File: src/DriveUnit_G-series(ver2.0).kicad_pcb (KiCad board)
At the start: 2 copper layers, 65.7 x 21.5 mm, 1 part

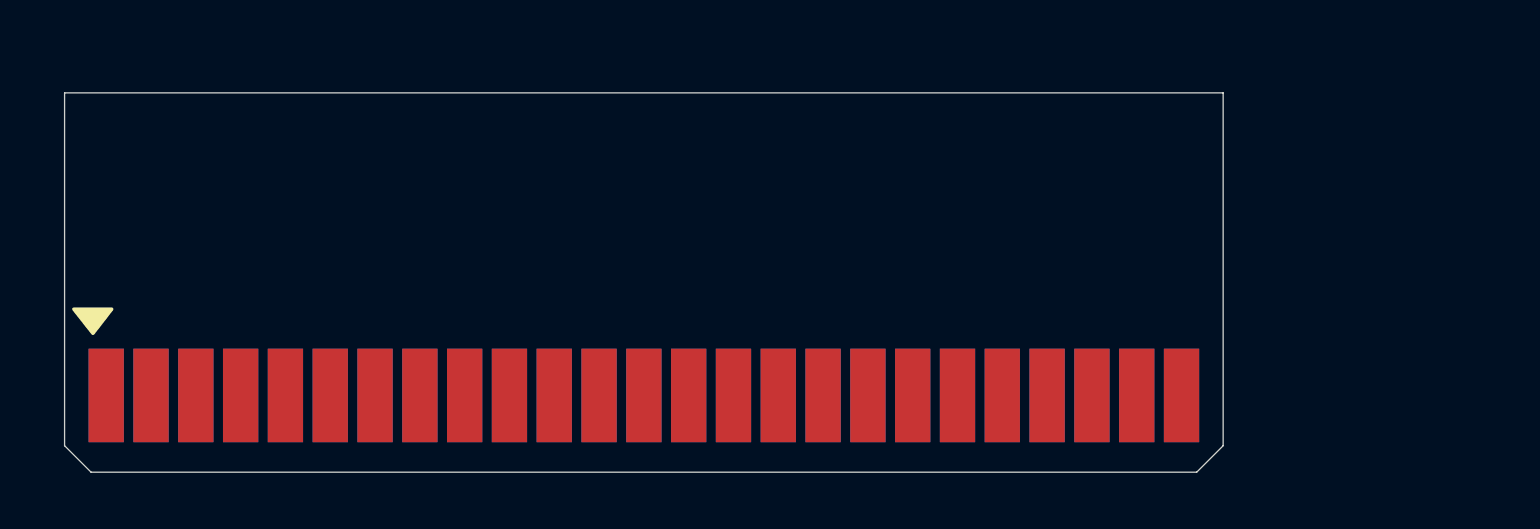
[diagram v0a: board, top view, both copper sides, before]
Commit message: [add]配線途中まで
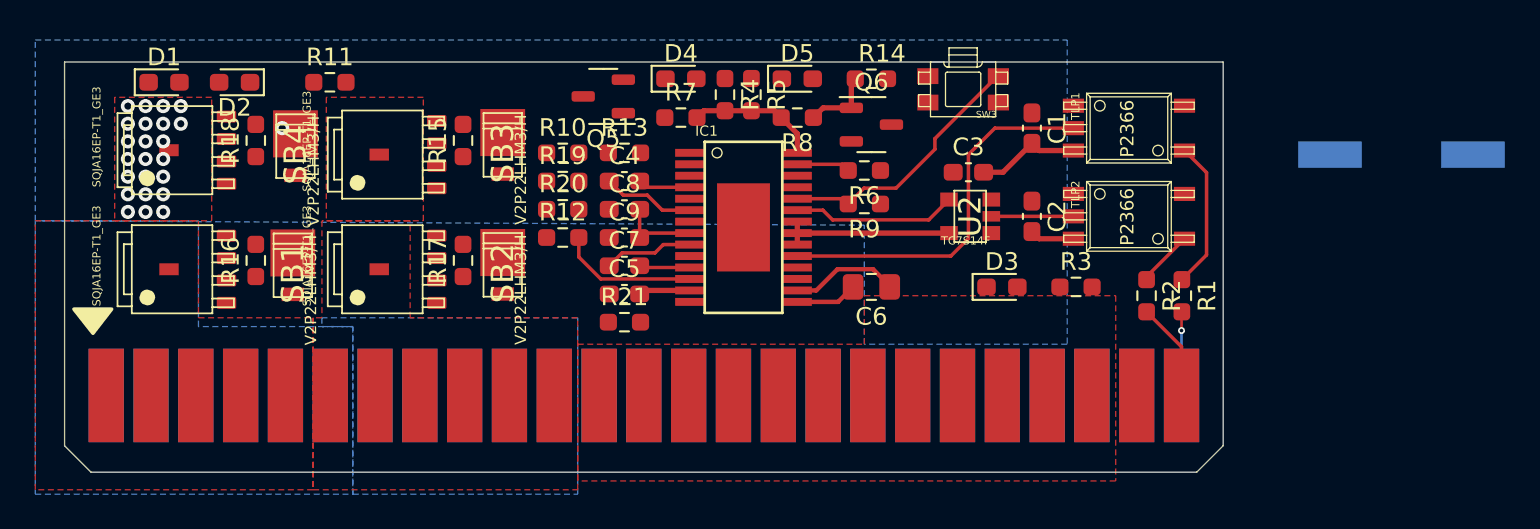
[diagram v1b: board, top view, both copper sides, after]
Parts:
- added C1: 100n, Capacitor_SMD:C_0603_1608Metric_Pad1.08x0.95mm_HandSolder, F.Cu at (170.5, 111.0)
- added C10: 220u, Symbol:U2-R_NCH, B.Cu at (191.4, 112.5)
- added C2: 100n, Capacitor_SMD:C_0603_1608Metric_Pad1.08x0.95mm_HandSolder, F.Cu at (170.5, 116.0)
- added C3: 100n, Capacitor_SMD:C_0603_1608Metric_Pad1.08x0.95mm_HandSolder, F.Cu at (166.9, 113.5)
- added C4: 100n, Capacitor_SMD:C_0603_1608Metric_Pad1.08x0.95mm_HandSolder, F.Cu at (147.4, 114.0)
- added C5: 100n, Capacitor_SMD:C_0603_1608Metric_Pad1.08x0.95mm_HandSolder, F.Cu at (147.4, 120.4)
- added C6: 470n, Capacitor_SMD:C_0805_2012Metric_Pad1.18x1.45mm_HandSolder, F.Cu at (161.4, 120.0)
- added C7: 100n, Capacitor_SMD:C_0603_1608Metric_Pad1.08x0.95mm_HandSolder, F.Cu at (147.4, 118.8)
- added C8: 100n, Capacitor_SMD:C_0603_1608Metric_Pad1.08x0.95mm_HandSolder, F.Cu at (147.4, 115.6)
- added C9: 2.2u, Capacitor_SMD:C_0603_1608Metric_Pad1.08x0.95mm_HandSolder, F.Cu at (147.4, 117.2)
- added D1: LED, LED_SMD:LED_0603_1608Metric_Pad1.05x0.95mm_HandSolder, F.Cu at (121.3, 108.4)
- added D2: LED, LED_SMD:LED_0603_1608Metric_Pad1.05x0.95mm_HandSolder, F.Cu at (125.3, 108.4)
- added D3: LED, LED_SMD:LED_0603_1608Metric_Pad1.05x0.95mm_HandSolder, F.Cu at (168.8, 120.0)
- added D4: LED, LED_SMD:LED_0603_1608Metric_Pad1.05x0.95mm_HandSolder, F.Cu at (150.6, 108.2)
- added D5: LED, LED_SMD:LED_0603_1608Metric_Pad1.05x0.95mm_HandSolder, F.Cu at (157.2, 108.2)
- added IC1: A3921, Symbol:A3921, F.Cu at (152.0, 112.4)
- added Q1: SQJA16EP-T1_GE3, Symbol:SQJA16EP-T1_GE3, F.Cu at (134.8, 112.5)
- added Q2: SQJA16EP-T1_GE3, Symbol:SQJA16EP-T1_GE3, F.Cu at (122.8, 119.0)
- added Q3: SQJA16EP-T1_GE3, Symbol:SQJA16EP-T1_GE3, F.Cu at (122.8, 112.2)
- added Q4: SQJA16EP-T1_GE3, Symbol:SQJA16EP-T1_GE3, F.Cu at (134.8, 119.0)
- added Q5: Q_NPN_BCE, Package_TO_SOT_SMD:SOT-23-3, F.Cu at (146.2, 109.2)
- added Q6: Q_NPN_BCE, Package_TO_SOT_SMD:SOT-23-3, F.Cu at (161.4, 110.8)
- added R1: 200, Resistor_SMD:R_0603_1608Metric_Pad0.98x0.95mm_HandSolder, F.Cu at (179.0, 120.5)
- added R10: 10, Resistor_SMD:R_0603_1608Metric_Pad0.98x0.95mm_HandSolder, F.Cu at (143.9, 112.4)
- added R11: 1k, Resistor_SMD:R_0603_1608Metric_Pad0.98x0.95mm_HandSolder, F.Cu at (130.7, 108.4)
- added R12: 10, Resistor_SMD:R_0603_1608Metric_Pad0.98x0.95mm_HandSolder, F.Cu at (143.9, 117.2)
- added R13: 100k, Resistor_SMD:R_0603_1608Metric_Pad0.98x0.95mm_HandSolder, F.Cu at (147.4, 112.4)
- added R14: 100k, Resistor_SMD:R_0603_1608Metric_Pad0.98x0.95mm_HandSolder, F.Cu at (161.4, 108.2)
- added R15: 10k, Resistor_SMD:R_0603_1608Metric_Pad0.98x0.95mm_HandSolder, F.Cu at (138.2, 111.7)
- added R16: 10k, Resistor_SMD:R_0603_1608Metric_Pad0.98x0.95mm_HandSolder, F.Cu at (126.5, 118.5)
- added R17: 10k, Resistor_SMD:R_0603_1608Metric_Pad0.98x0.95mm_HandSolder, F.Cu at (138.2, 118.5)
- added R18: 10k, Resistor_SMD:R_0603_1608Metric_Pad0.98x0.95mm_HandSolder, F.Cu at (126.5, 111.7)
- added R19: 10, Resistor_SMD:R_0603_1608Metric_Pad0.98x0.95mm_HandSolder, F.Cu at (143.9, 114.0)
- added R2: 200, Resistor_SMD:R_0603_1608Metric_Pad0.98x0.95mm_HandSolder, F.Cu at (177.0, 120.5)
- added R20: 10, Resistor_SMD:R_0603_1608Metric_Pad0.98x0.95mm_HandSolder, F.Cu at (143.9, 115.6)
- added R21: 10k, Resistor_SMD:R_0603_1608Metric_Pad0.98x0.95mm_HandSolder, F.Cu at (147.4, 122.0)
- added R3: 1k, Resistor_SMD:R_0603_1608Metric_Pad0.98x0.95mm_HandSolder, F.Cu at (173.0, 120.0)
- added R4: 200, Resistor_SMD:R_0603_1608Metric_Pad0.98x0.95mm_HandSolder, F.Cu at (153.1, 109.1)
- added R5: 200, Resistor_SMD:R_0603_1608Metric_Pad0.98x0.95mm_HandSolder, F.Cu at (154.6, 109.1)
- added R6: 3k, Resistor_SMD:R_0603_1608Metric_Pad0.98x0.95mm_HandSolder, F.Cu at (161.0, 113.4)
- added R7: 10k, Resistor_SMD:R_0603_1608Metric_Pad0.98x0.95mm_HandSolder, F.Cu at (150.6, 110.4)
- added R8: 10k, Resistor_SMD:R_0603_1608Metric_Pad0.98x0.95mm_HandSolder, F.Cu at (157.2, 110.4)
- added R9: 10k, Resistor_SMD:R_0603_1608Metric_Pad0.98x0.95mm_HandSolder, F.Cu at (161.0, 115.3)
- added SB1: V2P22LHM3/H, Symbol:V2P22LHM3_H, F.Cu at (128.6, 119.2)
- added SB2: V2P22LHM3/H, Symbol:V2P22LHM3_H, F.Cu at (140.5, 119.2)
- added SB3: V2P22LHM3/H, Symbol:V2P22LHM3_H, F.Cu at (140.5, 112.4)
- added SB4: V2P22LHM3/H, Symbol:V2P22LHM3_H, F.Cu at (128.8, 112.5)
- added SW3: THAF01-NC-R, Symbol:THAF01-NC-R, F.Cu at (168.6, 108.0)
- added TLP1: TLP2366, Symbol:TLP2366, F.Cu at (179.2, 112.3)
- added TLP2: TLP2366, Symbol:TLP2366, F.Cu at (179.2, 117.3)
- added U2: TC7S14F, Symbol:TC7S14F, F.Cu at (167.0, 116.0)
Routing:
- net /V5: track 0.00 -> 25.8 mm
- net /DIR: track 0.00 -> 21.4 mm
- net /RESET: track 0.00 -> 14.9 mm
- net /PWM: track 0.00 -> 9.30 mm
- net Net-(TLP1-ANODE): track 0.00 -> 8.42 mm
- net /GLA: track 0.00 -> 7.91 mm
- net Net-(IC1-CP1): track 0.00 -> 6.19 mm
- net /PWM_IN: track 0.00 -> 5.56 mm
- net Net-(IC1-CB): track 0.00 -> 5.25 mm
- net Net-(IC1-CA): track 0.00 -> 5.06 mm
- net Net-(TLP2-VOUT): track 0.00 -> 4.65 mm
- net Net-(IC1-VREG): track 0.00 -> 4.54 mm
- net /FF2: track 0.00 -> 4.12 mm
- net Net-(IC1-CP2): track 0.00 -> 3.51 mm
- net Net-(TLP2-ANODE): track 0.00 -> 3.21 mm
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- added copper zone on B.Cu, net /SA
- added copper zone on F.Cu, net /SA
- added copper zone on B.Cu, net /SB
- added copper zone on F.Cu, net /SB
- added copper zone on B.Cu, net VCC
- added copper zone on F.Cu, net VCC
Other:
- board size 65.7 x 21.5 mm -> 65.7 x 23.3 mm
